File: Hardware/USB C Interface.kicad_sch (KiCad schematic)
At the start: 5 parts, among them J2 USB_C_Receptacle_USB2.0, U14 TPD4E02B04DQA

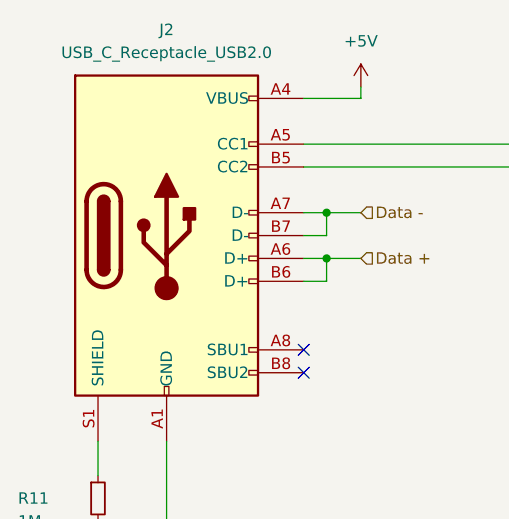
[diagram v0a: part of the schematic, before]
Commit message: BIG Changes
Create a 4 Layer Variation
Change Motor Controller routing.
Change Power Regulation.
Optimize Sensor routing.
Pray I know what i'm doing
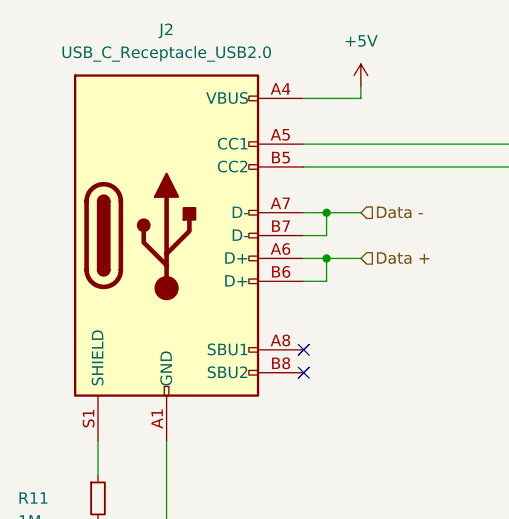
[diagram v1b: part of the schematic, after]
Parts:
- J2: footprint Connector_USB:USB_C_Receptacle_XKB_U262-16XN-4BVC11 -> Connector_USB:USB_C_Receptacle_GCT_USB4110
- R11, R12, R13: footprint Resistor_SMD:R_0805_2012Metric -> Resistor_SMD:R_0603_1608Metric
